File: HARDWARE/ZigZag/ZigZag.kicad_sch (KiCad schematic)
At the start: 42 parts, among them SW1 SW_Push, T1 2N3904, U1 CH32V003J4M6(SOP8)

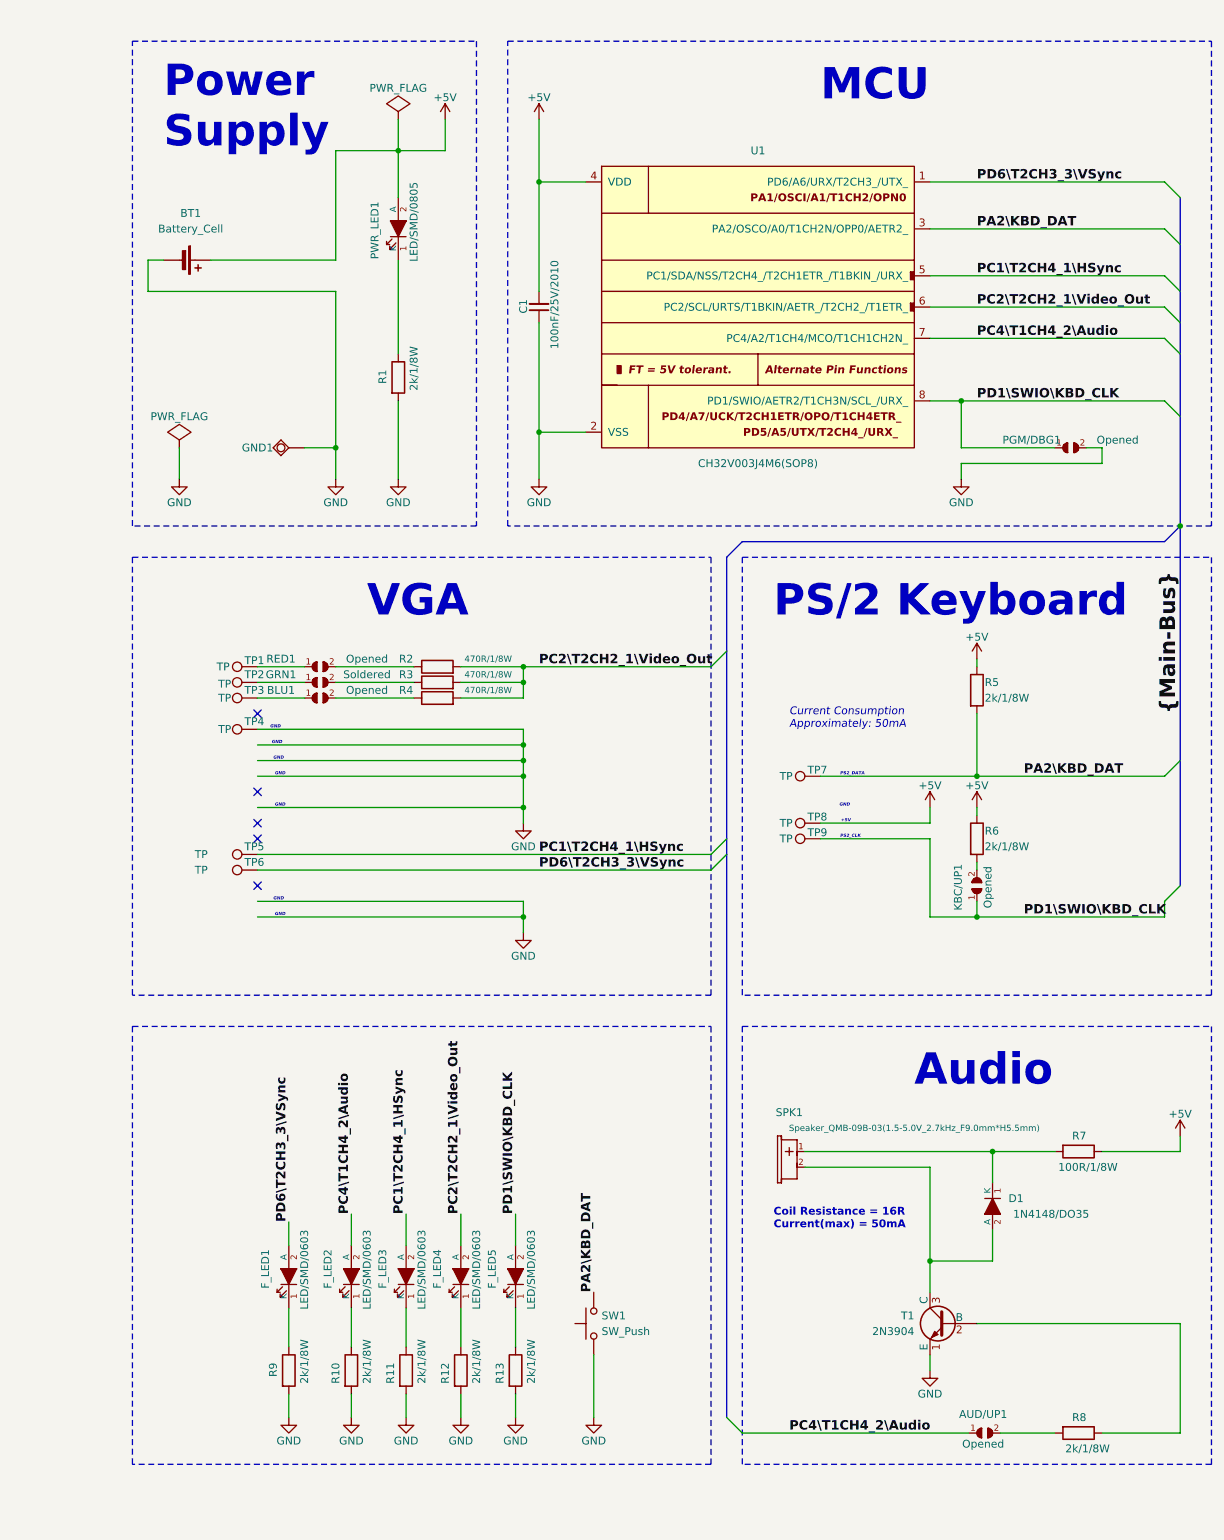
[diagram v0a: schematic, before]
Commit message: uređena schema
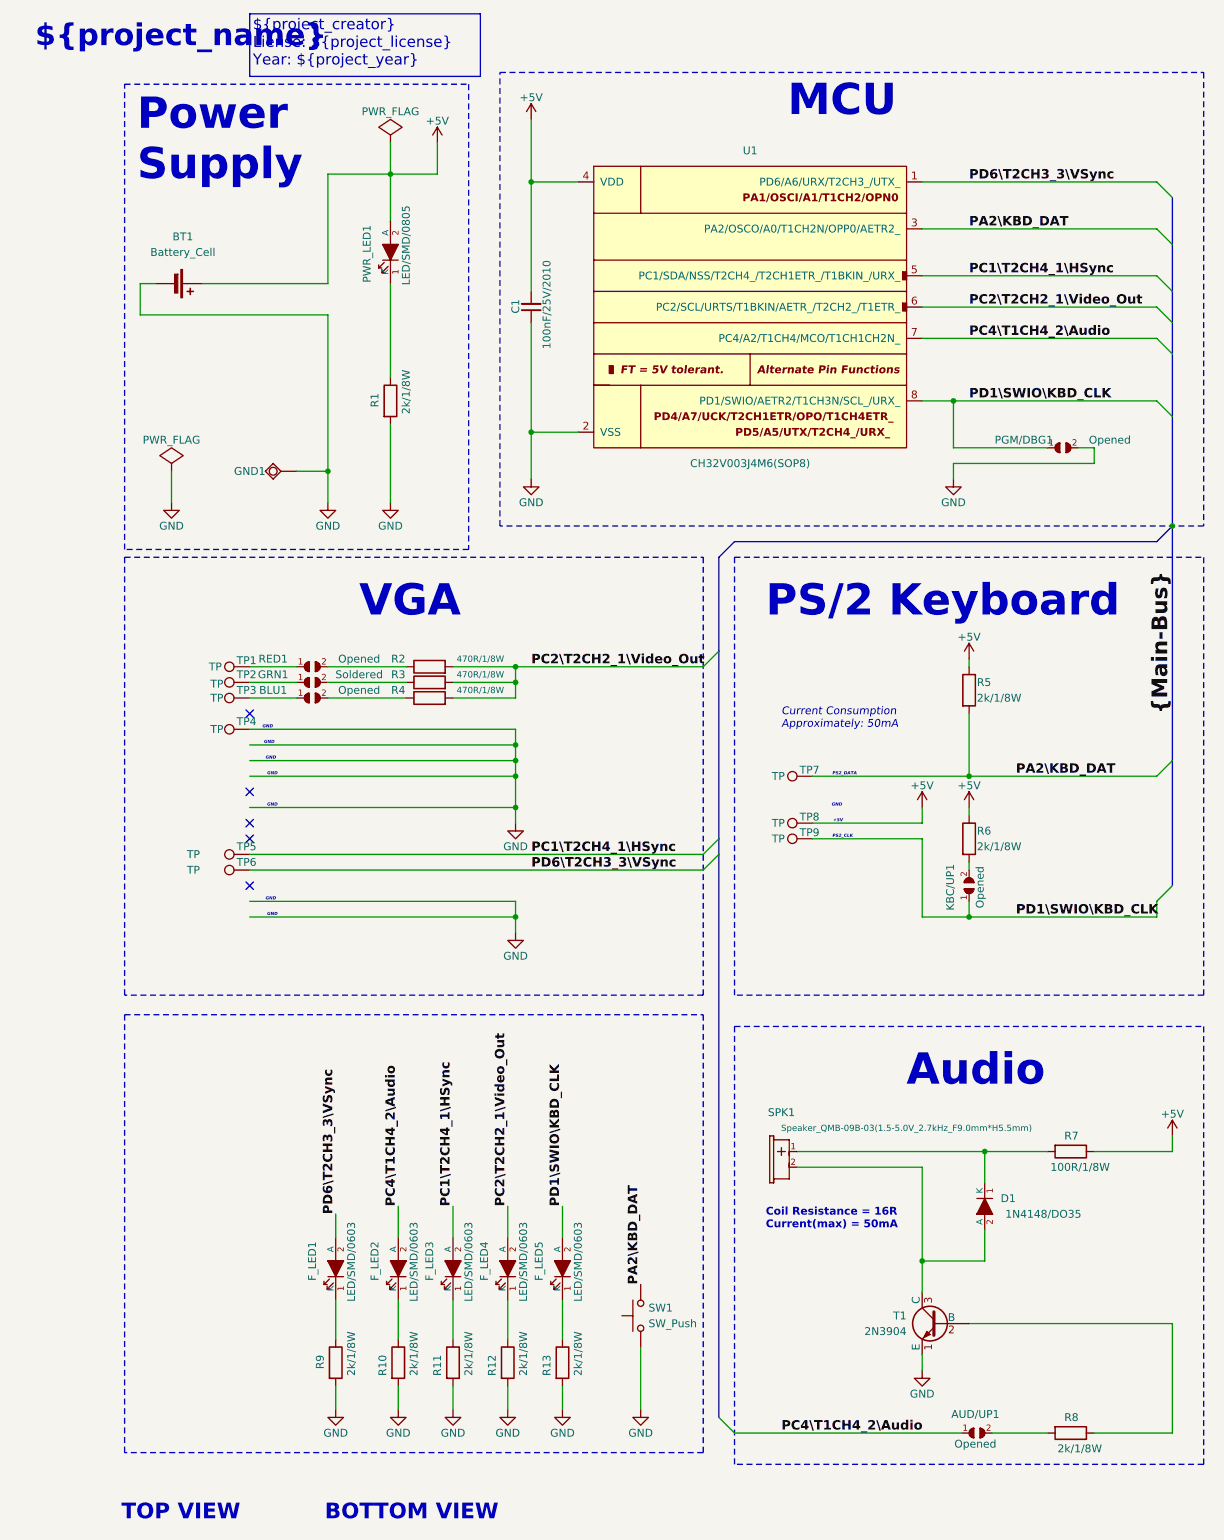
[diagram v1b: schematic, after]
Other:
- note added: "${project_creator} Liense: ${project_license} Year: ${project_year}"
- note added: "${project_name}"
- note added: "BOTTOM VIEW"
- note added: "TOP VIEW"
- company: Radiona Org -> ${project_creator}
- title: ZagZag -> ${project_name} ${project_version}
- moved on the sheet: AUD/UP1, BLU1, BT1, C1, D1, F_LED1, F_LED2, F_LED3, F_LED4, F_LED5, GND1, GRN1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
